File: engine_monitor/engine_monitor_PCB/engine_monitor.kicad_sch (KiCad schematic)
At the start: 39 parts, among them J1 temp_1, J2 temp_2, J3 temp_3, J4 PWR_in, J5 SW_Fan_GND, J6 rs-485, J7 temp_4, J8 O2_sensor, Q1 IRLS3036, U1 ATtiny3216-S, U2 AP63205WU, U3 AP2112K-3.3, U4 MCP1406-E/SN, U5 THVD1420D

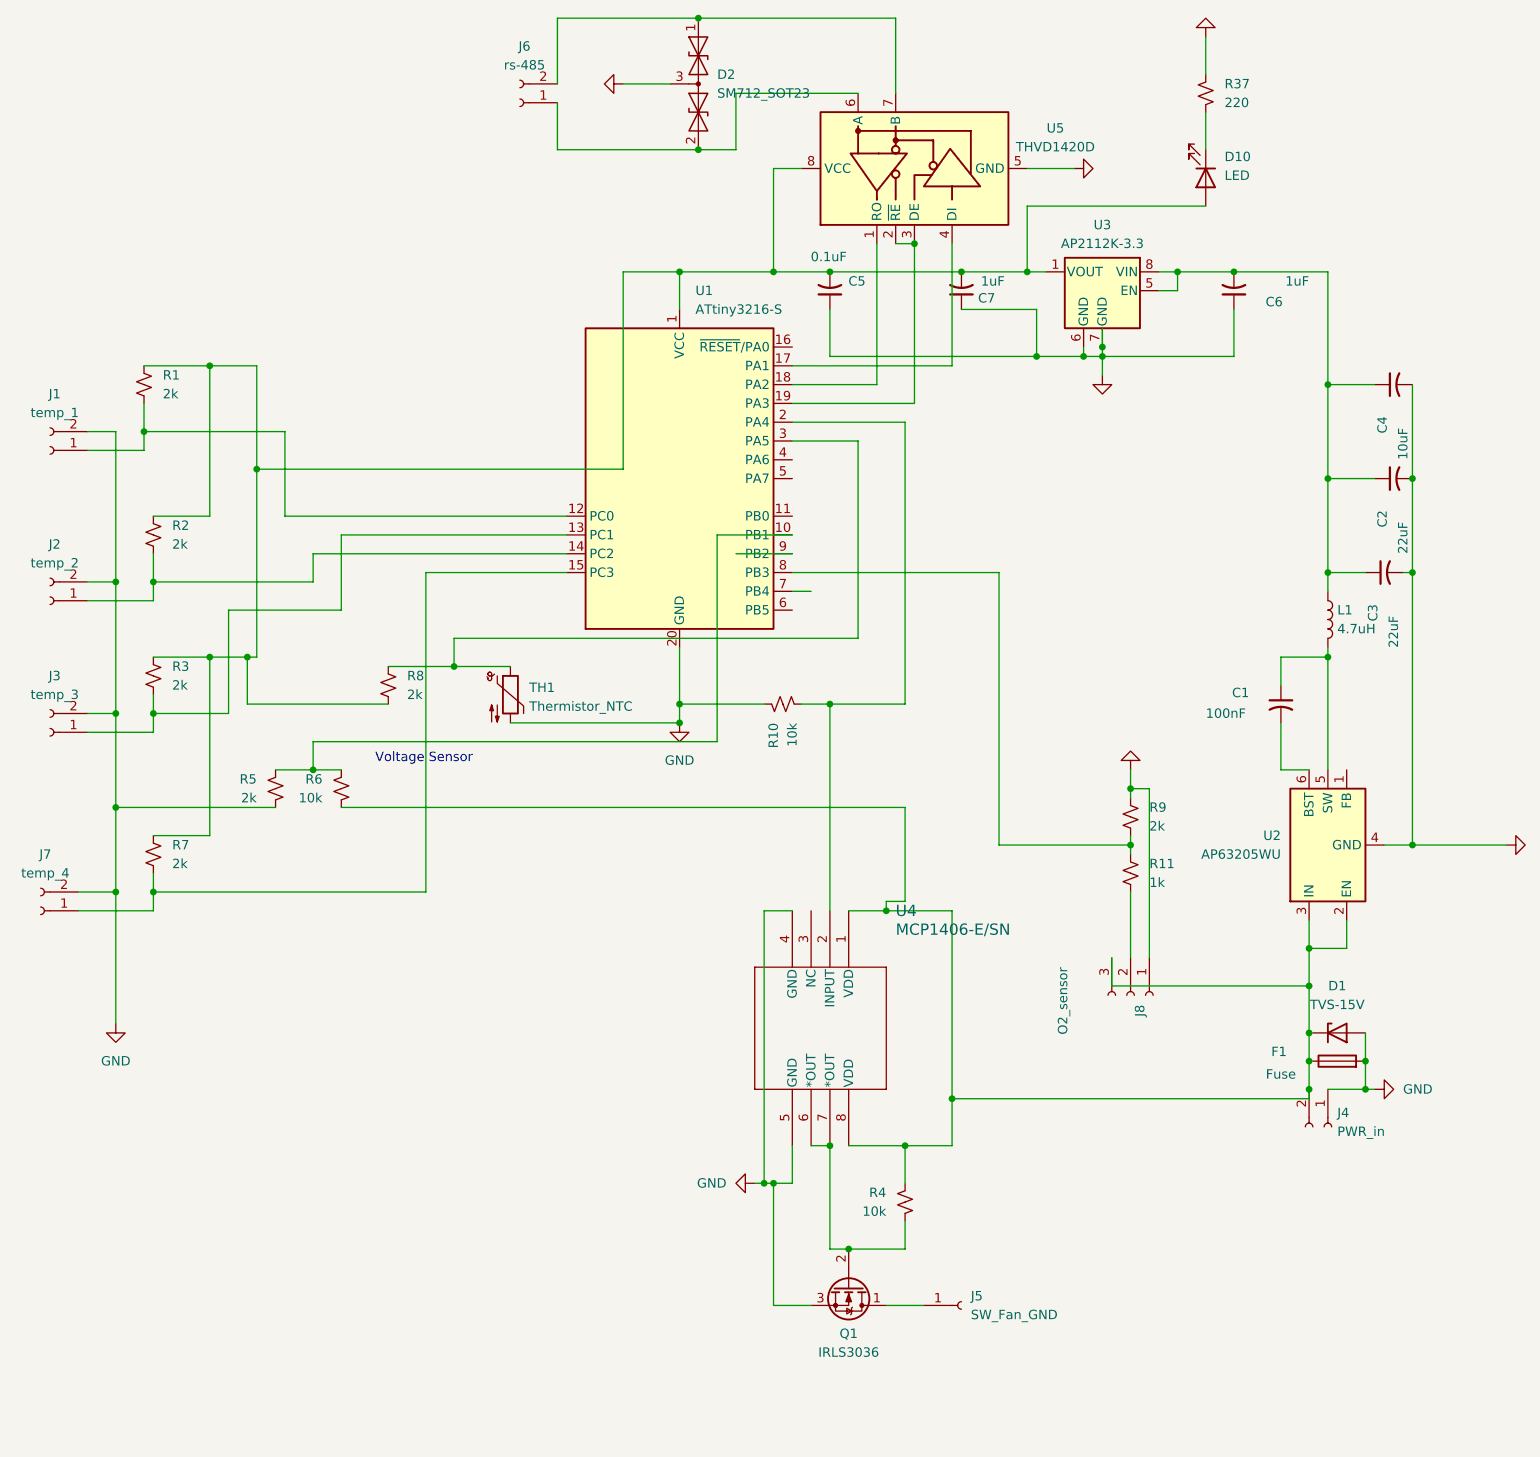
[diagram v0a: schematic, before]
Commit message: project progress
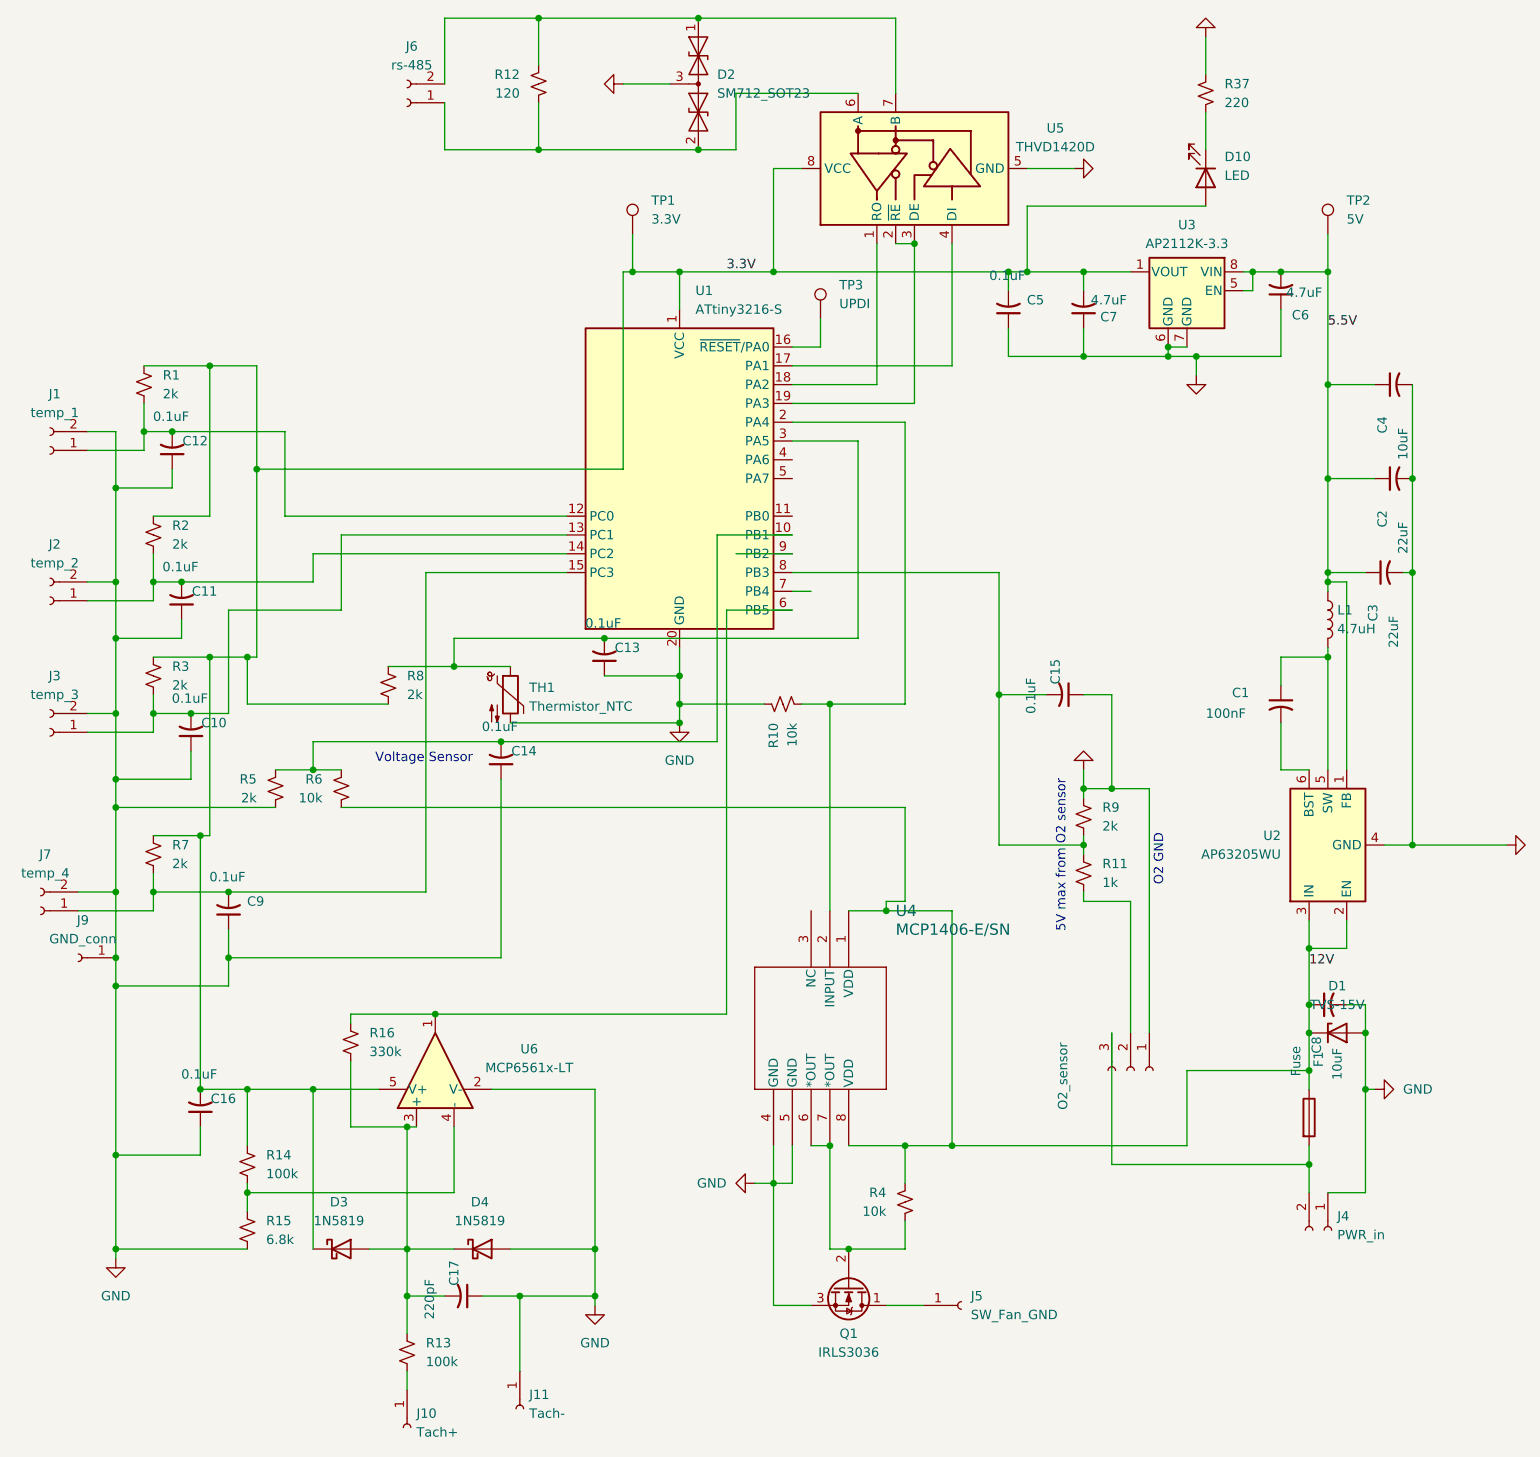
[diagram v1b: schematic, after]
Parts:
- added C10, C11, C12, C13, C14, C15, C16, C9: 0.1uF, Capacitor_SMD:C_1206_3216Metric_Pad1.33x1.80mm_HandSolder, symbol Device:C_Small_US
- added C17: 220pF, Capacitor_SMD:C_1206_3216Metric_Pad1.33x1.80mm_HandSolder, symbol Device:C_Small_US
- added C8: 10uF, Capacitor_SMD:C_1206_3216Metric_Pad1.33x1.80mm_HandSolder, symbol Device:C_Small_US
- added D3, D4: 1N5819, Diode_SMD:D_SOD-123, symbol Diode:1N5819
- added J10: Tach+, Connector:Alex_1pin_065thou, symbol Connector:Conn_01x01_Socket
- added J11: Tach-, Connector:Alex_1pin_065thou, symbol Connector:Conn_01x01_Socket
- added J9: GND_conn, Connector:Alex_1pin_065thou, symbol Connector:Conn_01x01_Socket
- added R12: 120, Resistor_SMD:R_1206_3216Metric_Pad1.30x1.75mm_HandSolder, symbol Device:R_Small_US
- added R13, R14: 100k, Resistor_SMD:R_1206_3216Metric_Pad1.30x1.75mm_HandSolder, symbol Device:R_Small_US
- added R15: 6.8k, Resistor_SMD:R_1206_3216Metric_Pad1.30x1.75mm_HandSolder, symbol Device:R_Small_US
- added R16: 330k, Resistor_SMD:R_1206_3216Metric_Pad1.30x1.75mm_HandSolder, symbol Device:R_Small_US
- added TP1: 3.3V, TestPoint:TestPoint_Pad_2.5x2.5mm, symbol Connector:TestPoint
- added TP2: 5V, TestPoint:TestPoint_Pad_2.5x2.5mm, symbol Connector:TestPoint
- added TP3: UPDI, TestPoint:TestPoint_Pad_2.5x2.5mm, symbol Connector:TestPoint
- added U6: MCP6561x-LT, Package_TO_SOT_SMD:SOT-23-5, symbol Comparator:MCP6561x-LT
- C6, C7: value 1uF -> 4.7uF
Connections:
- net GND: now also C10.1, C11.1, C12.1, C13.1, C14.1, C15.1, C16.1, C17.1, C8.2, C9.1, D4.2 (A), J11.1 (Pin_1), J9.1 (Pin_1), R15.2, U6.2 (V-); no longer F1.2
- net at D2.2 (A2), J6.1 (Pin_1), U5.6 (A): now also R12.2
- net at D2.1 (A1), J6.2 (Pin_2), U5.7 (B): now also R12.1
- net 3.3V: now reaches C5.2, C7.2, D10.2 (A), R1.1, R2.1, R3.1, R7.1, R8.2, U1.1 (VCC), U3.1 (VOUT), U5.8 (VCC)
- net 3.3V: now also C16.2, D3.1 (K), R14.1, TP1.1, U6.5 (V+)
- net 5.5V: now reaches C2.1, C3.1, C4.1, C6.2, L1.1, U3.5 (EN), U3.8 (VIN)
- net 5.5V: now also U2.1 (FB), TP2.1
- net at J3.1 (Pin_1), R3.2, U1.13 (PC1): now also C10.2
- net at R5.1, R6.1, U1.10 (PB1): now also C14.2
- net 12V: now reaches D1.1 (K), F1.1, R4.1, R6.2, U2.2 (EN), U2.3 (IN), U4.1 (VDD), U4.8 (VDD)
- net 12V: now also C8.1; no longer J4.2 (Pin_2), J8.3 (Pin_3)
- net at J1.1 (Pin_1), R1.2, U1.12 (PC0): now also C12.2
- net at J2.1 (Pin_1), R2.2, U1.14 (PC2): now also C11.2
- net at J7.1 (Pin_1), R7.2, U1.15 (PC3): now also C9.2
- net at U1.16 (~{RESET}/PA0): now also TP3.1
- net at R8.1, TH1.1, U1.3 (PA5): now also C13.2
- net at U1.6 (PB5): now also R16.1, U6.1
- net at R11.1, R9.2, U1.8 (PB3): now also C15.2
- new net: C17.2, D3.2 (A), D4.1 (K), R13.1, R16.2, U6.3 (+)
- new net: R14.2, R15.1, U6.4 (-)
- new net: J10.1 (Pin_1), R13.2
- new net: F1.2, J4.2 (Pin_2), J8.3 (Pin_3)
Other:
- note added: "5V max from O2 sensor"
- note added: "O2 GND"
- moved on the sheet: C5, C6, C7, F1, J4, J6, R11, R9, U3

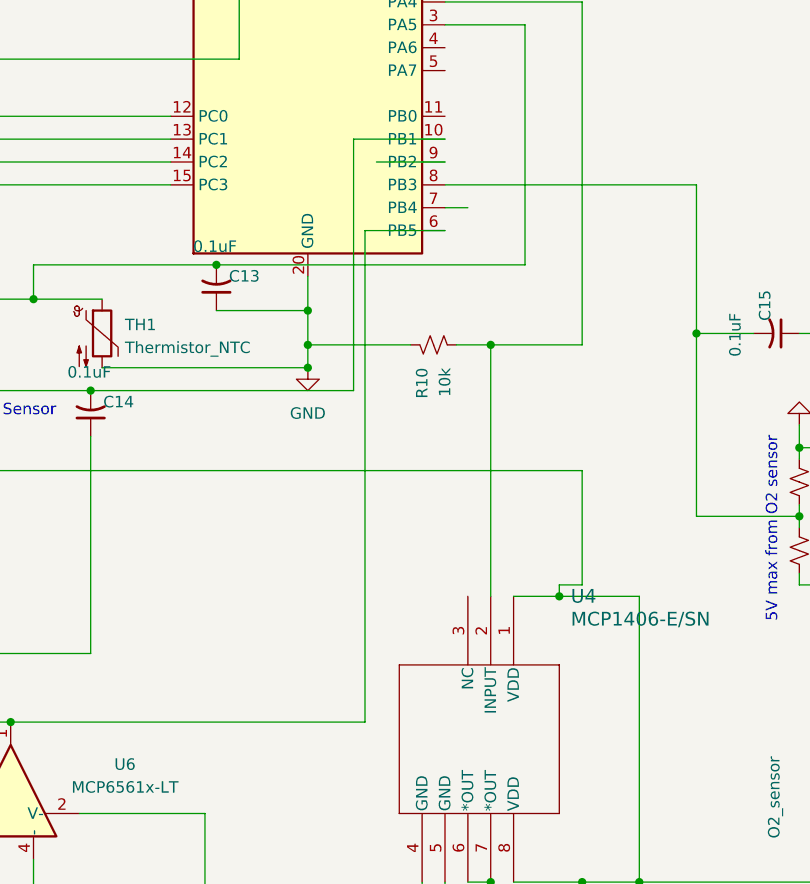
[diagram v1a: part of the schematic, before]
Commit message: layout for the day
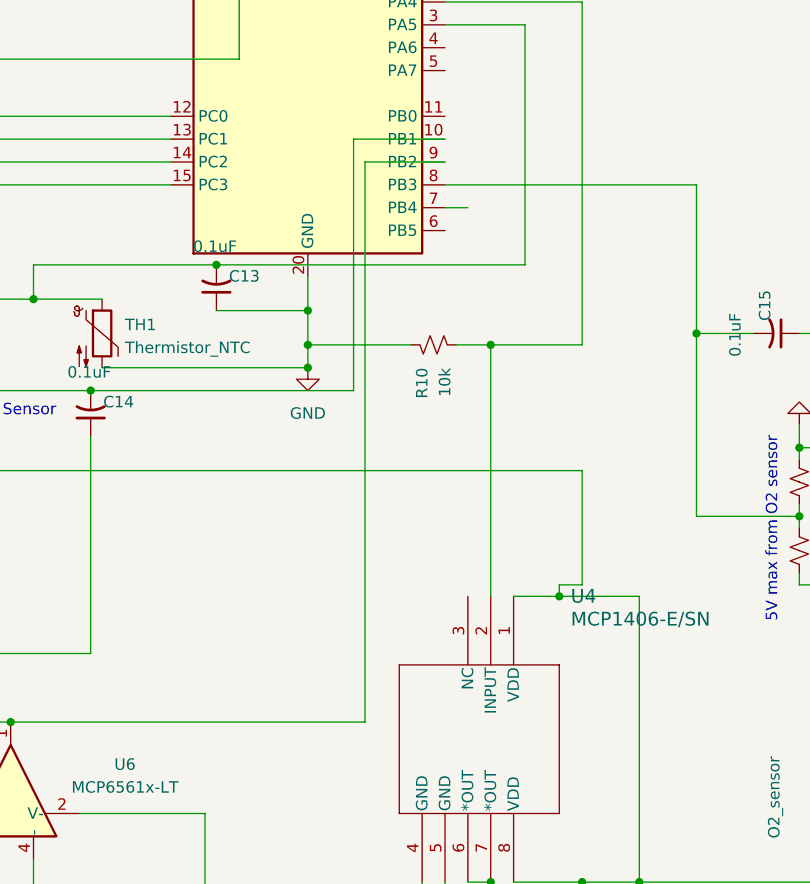
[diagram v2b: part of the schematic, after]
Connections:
- net at R16.1, U6.1: now also U1.9 (PB2); no longer U1.6 (PB5)
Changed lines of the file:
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@@
+	(wire
+		(pts
+			(xy 109.22 86.36) (xy 118.11 86.36)
+		)
+		(stroke
+			(width 0)
+			(type default)
+		)
+	)
 	(wire
 		(pts
@@
 	(wire
 		(pts
-			(xy 110.49 86.36) (xy 118.11 86.36)
-		)
-		(stroke
-			(width 0)
-			(type default)
-		)
-	)
-	(wire
-		(pts
 			(xy 66.04 163.83) (xy 67.31 163.83)
 		)
@@
 	(wire
 		(pts
+			(xy 109.22 86.36) (xy 109.22 148.59)
+		)
+		(stroke
+			(width 0)
+			(type default)
+		)
+	)
+	(wire
+		(pts
 			(xy 118.11 63.5) (xy 129.54 63.5)
 		)
@@
 	(wire
 		(pts
-			(xy 118.11 93.98) (xy 109.22 93.98)
-		)
-		(stroke
-			(width 0)
-			(type default)
-		)
-	)
-	(wire
-		(pts
 			(xy 38.1 124.46) (xy 38.1 158.75)
 		)
@@
 		)
 		(stroke
-			(width 0)
-			(type default)
-		)
-	)
-	(wire
-		(pts
-			(xy 109.22 93.98) (xy 109.22 148.59)
-		)
-		(stroke
